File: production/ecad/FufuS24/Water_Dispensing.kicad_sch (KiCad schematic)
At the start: 8 parts, among them J12 691137710002, J13 5033950410, J8 691137710004, Q1 DMG2302UK-7

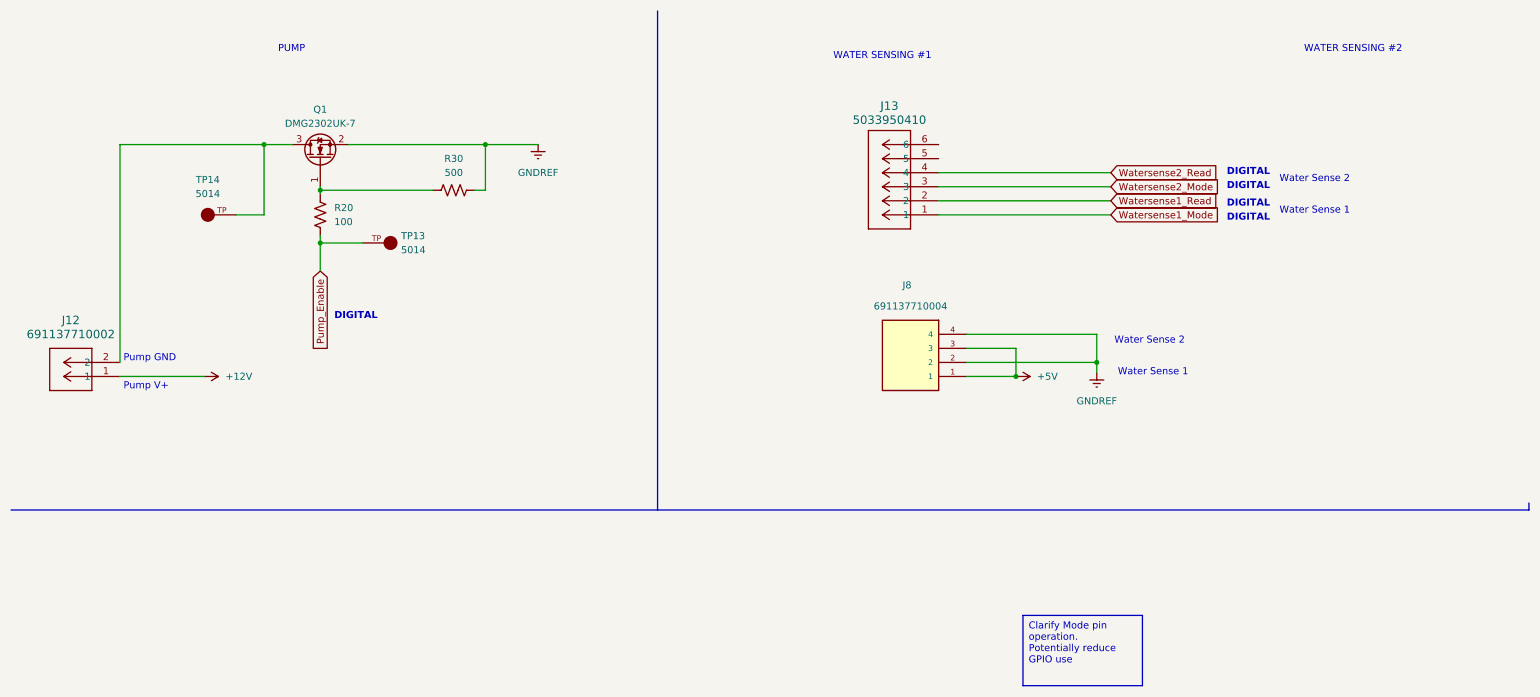
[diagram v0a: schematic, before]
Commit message: Big layout push
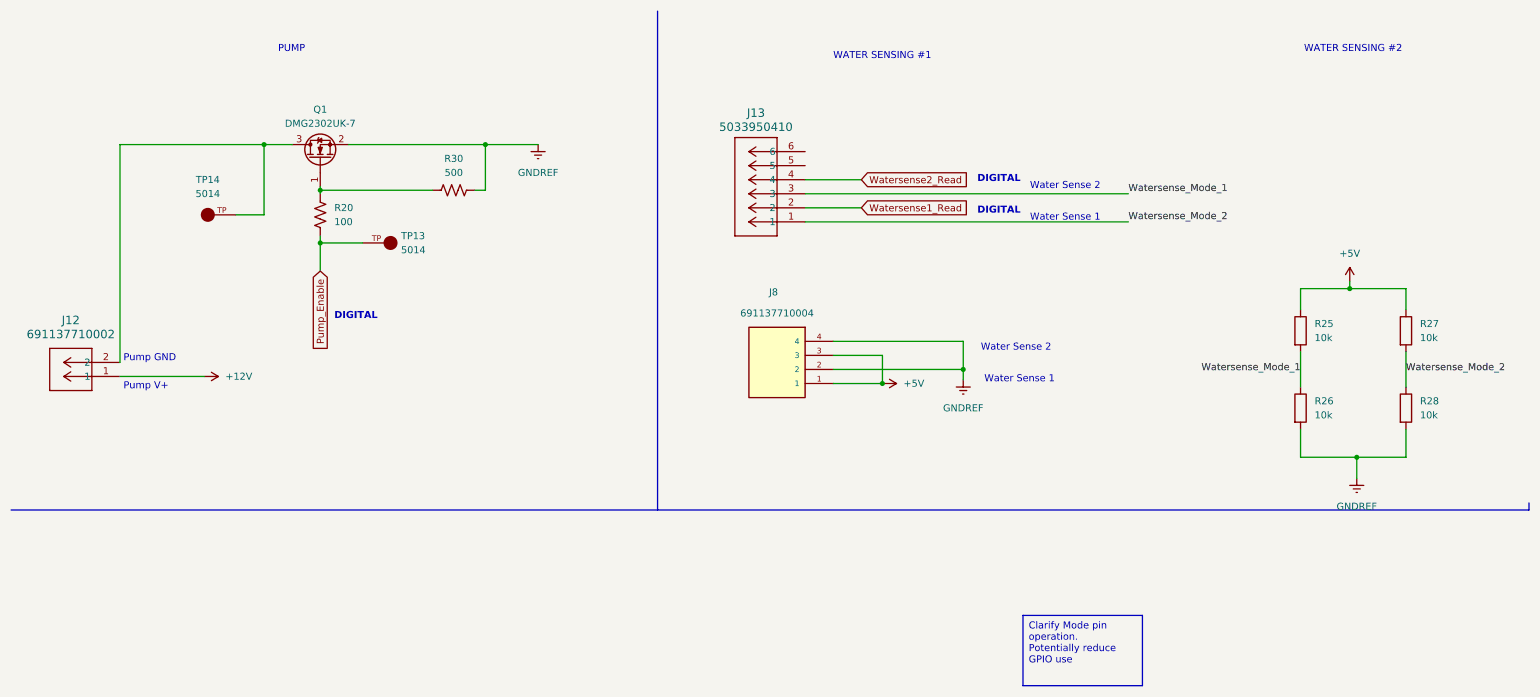
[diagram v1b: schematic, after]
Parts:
- added R25, R26, R27, R28: 10k, footprints:RESC2012X60N, symbol Device:R
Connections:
- net +5V: now also R25.1, R27.1
- net GNDREF: now also R26.2, R28.2
- net Watersense1_Mode renamed Watersense_Mode_2
- net Watersense_Mode_2: now also R27.2, R28.1
- net Watersense2_Mode renamed Watersense_Mode_1
- net Watersense_Mode_1: now also R25.2, R26.1
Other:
- moved on the sheet: J13, J8
